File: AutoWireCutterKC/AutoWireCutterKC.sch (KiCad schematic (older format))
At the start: 8 parts, among them J1 LCD I/O, J2 ISP, J3 LCD Serial, J4 Conn_02x08_Top_Bottom, J5 Stepper

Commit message: Schematic Finished
TODO: Double check connections
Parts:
- added C3, C4, C5: 1u, symbol C
- added C6: 3.3u, symbol CP1
- added J6: LCD Power, symbol Conn_01x03
- added J7: Servo, symbol Conn_01x03
- added J7: Barrel_Jack, symbol Barrel_Jack
- added U2: MCP1700_SOT23, TO_SOT_Packages_SMD:SOT-23, symbol MCP1700-5002E_SOT23
- added U3: LT1129-5.0_SOT223, TO_SOT_Packages_SMD:SOT-223-3Lead_TabPin2, symbol LT1129-5.0_SOT223
- gave numbers to parts that had none: 1
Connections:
- net labels added: +12V, +5V, +5VL
- net labels removed: +24V
- wire segments 80 -> 110
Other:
- moved on the sheet: C1, C2, J1, J2, J3, J4, J5, U1

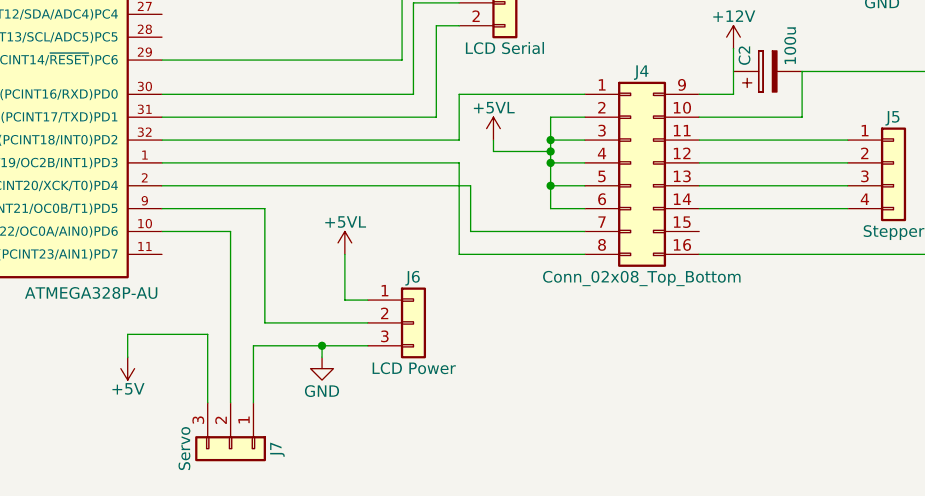
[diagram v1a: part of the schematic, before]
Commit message: Working on footprints
in progress
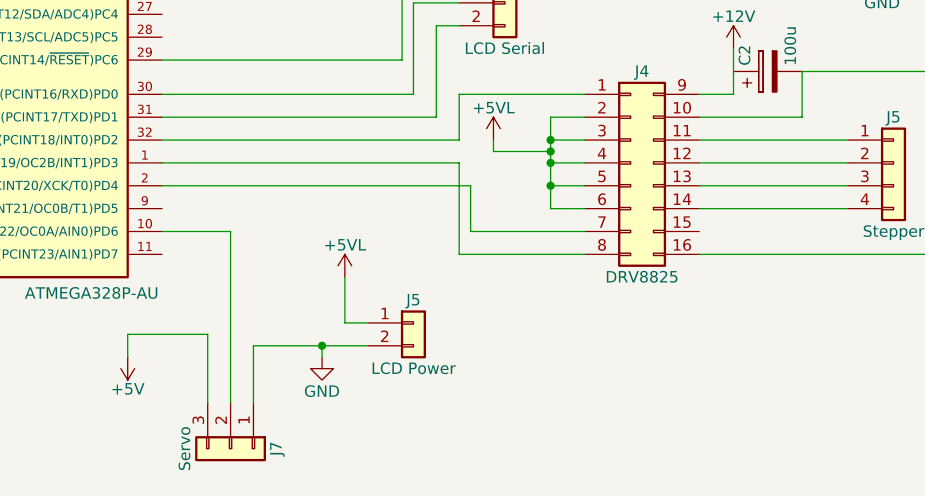
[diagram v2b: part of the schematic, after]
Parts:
- removed J6: LCD Power, symbol Conn_01x03
- added J5: LCD Power, Pin_Headers:Pin_Header_Angled_1x02_Pitch2.54mm, symbol Conn_01x02
- J2: footprint (none) -> Pin_Headers:Pin_Header_Straight_2x03_Pitch2.54mm
- J3: footprint (none) -> Pin_Headers:Pin_Header_Angled_1x02_Pitch2.54mm
- J4: value Conn_02x08_Top_Bottom -> DRV8825
- J5: footprint (none) -> Pin_Headers:Pin_Header_Straight_1x04_Pitch2.54mm
- J7: footprint (none) -> Pin_Headers:Pin_Header_Angled_1x03_Pitch2.54mm
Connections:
- net +5VL: now also J5.1 (Pin_1)
- net GND: now also J5.2 (Pin_2)
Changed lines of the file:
@@
 F 0 "J3" H 4950 4050 50  0000 C CNN
 F 1 "LCD Serial" H 4950 3750 50  0000 C CNN
-F 2 "" H 4950 3950 50  0001 C CNN
+F 2 "Pin_Headers:Pin_Header_Angled_1x02_Pitch2.54mm" H 4950 3950 50  0001 C CNN
 F 3 "" H 4950 3950 50  0001 C CNN
 	1    4950 3950
@@
 F 0 "J2" H 6200 3800 50  0000 C CNN
 F 1 "ISP" H 6200 3400 50  0000 C CNN
-F 2 "" H 6150 3600 50  0001 C CNN
+F 2 "Pin_Headers:Pin_Header_Straight_2x03_Pitch2.54mm" H 6150 3600 50  0001 C CNN
 F 3 "" H 6150 3600 50  0001 C CNN
 	1    6150 3600
@@
 P 5500 4650
 F 0 "J4" H 5550 5050 50  0000 C CNN
-F 1 "Conn_02x08_Top_Bottom" H 5550 4150 50  0000 C CNN
+F 1 "DRV8825" H 5550 4150 50  0000 C CNN
 F 2 "" H 5500 4650 50  0001 C CNN
 F 3 "" H 5500 4650 50  0001 C CNN
@@
 F 0 "J5" H 6650 4850 50  0000 C CNN
 F 1 "Stepper" H 6650 4350 50  0000 C CNN
-F 2 "" H 6650 4650 50  0001 C CNN
+F 2 "Pin_Headers:Pin_Header_Straight_1x04_Pitch2.54mm" H 6650 4650 50  0001 C CNN
 F 3 "" H 6650 4650 50  0001 C CNN
 	1    6650 4650
@@
 $EndComp
 $Comp
-L Conn_01x03 J6
-U 1 1 5B1A9FB3
-P 4550 5350
-F 0 "J6" H 4550 5550 50  0000 C CNN
-F 1 "LCD Power" H 4550 5150 50  0000 C CNN
-F 2 "" H 4550 5350 50  0001 C CNN
-F 3 "" H 4550 5350 50  0001 C CNN
-	1    4550 5350
-	1    0    0    -1
-$EndComp
-$Comp
 L GND #PWR?
 U 1 1 5B1AA1E5
@@
 F 0 "J7" H 3750 6100 50  0000 C CNN
 F 1 "Servo" H 3750 5700 50  0000 C CNN
-F 2 "" H 3750 5900 50  0001 C CNN
+F 2 "Pin_Headers:Pin_Header_Angled_1x03_Pitch2.54mm" H 3750 5900 50  0001 C CNN
 F 3 "" H 3750 5900 50  0001 C CNN
 	1    3750 5900
@@
 	6950 5050 5800 5050
 Wire Wire Line
-	3450 4850 3900 4850
-Wire Wire Line
-	3900 4850 3900 5350
-Wire Wire Line
-	3900 5350 4350 5350
-Wire Wire Line
 	3850 5450 4350 5450
 Wire Wire Line
 	4150 5450 4150 5500
 Wire Wire Line
-	4250 5050 4250 5250
-Wire Wire Line
-	4250 5250 4350 5250
+	4250 5150 4250 5350
+Wire Wire Line
+	4250 5350 4350 5350
 Wire Wire Line
 	3450 4950 3750 4950
@@
 L +5VL #PWR?
 U 1 1 5B1EDDCC
-P 4250 5050
-F 0 "#PWR?" H 4250 4900 50  0001 C CNN
-F 1 "+5VL" H 4250 5190 50  0000 C CNN
-F 2 "" H 4250 5050 50  0001 C CNN
-F 3 "" H 4250 5050 50  0001 C CNN
-	1    4250 5050
+P 4250 5150
+F 0 "#PWR?" H 4250 5000 50  0001 C CNN
+F 1 "+5VL" H 4250 5290 50  0000 C CNN
+F 2 "" H 4250 5150 50  0001 C CNN
+F 3 "" H 4250 5150 50  0001 C CNN
+	1    4250 5150
 	1    0    0    -1
 $EndComp
@@
 	1    0    0    -1
 $EndComp
+$Comp
+L Conn_01x02 J5
+U 1 1 5B1EE683
+P 4550 5350
+F 0 "J5" H 4550 5450 50  0000 C CNN
+F 1 "LCD Power" H 4550 5150 50  0000 C CNN
+F 2 "Pin_Headers:Pin_Header_Angled_1x02_Pitch2.54mm" H 4550 5350 50  0001 C CNN
+F 3 "" H 4550 5350 50  0001 C CNN
+	1    4550 5350
+	1    0    0    -1
+$EndComp
